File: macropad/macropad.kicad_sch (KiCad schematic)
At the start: 7 parts, among them SW1 SW_Push, SW2 SW_Push, SW3 SW_Push, SW4 SW_Push, U1 XIAO-RP2040-DIP

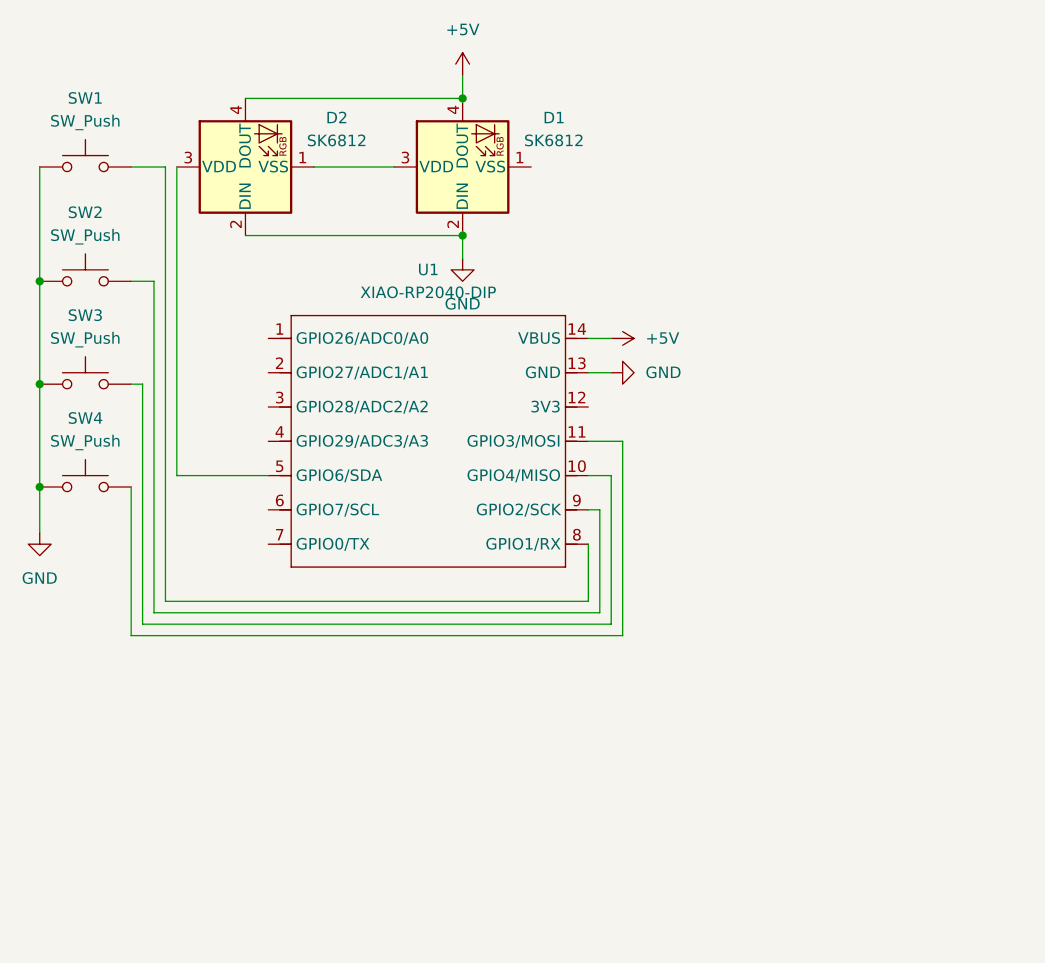
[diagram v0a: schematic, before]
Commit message: Add files via upload
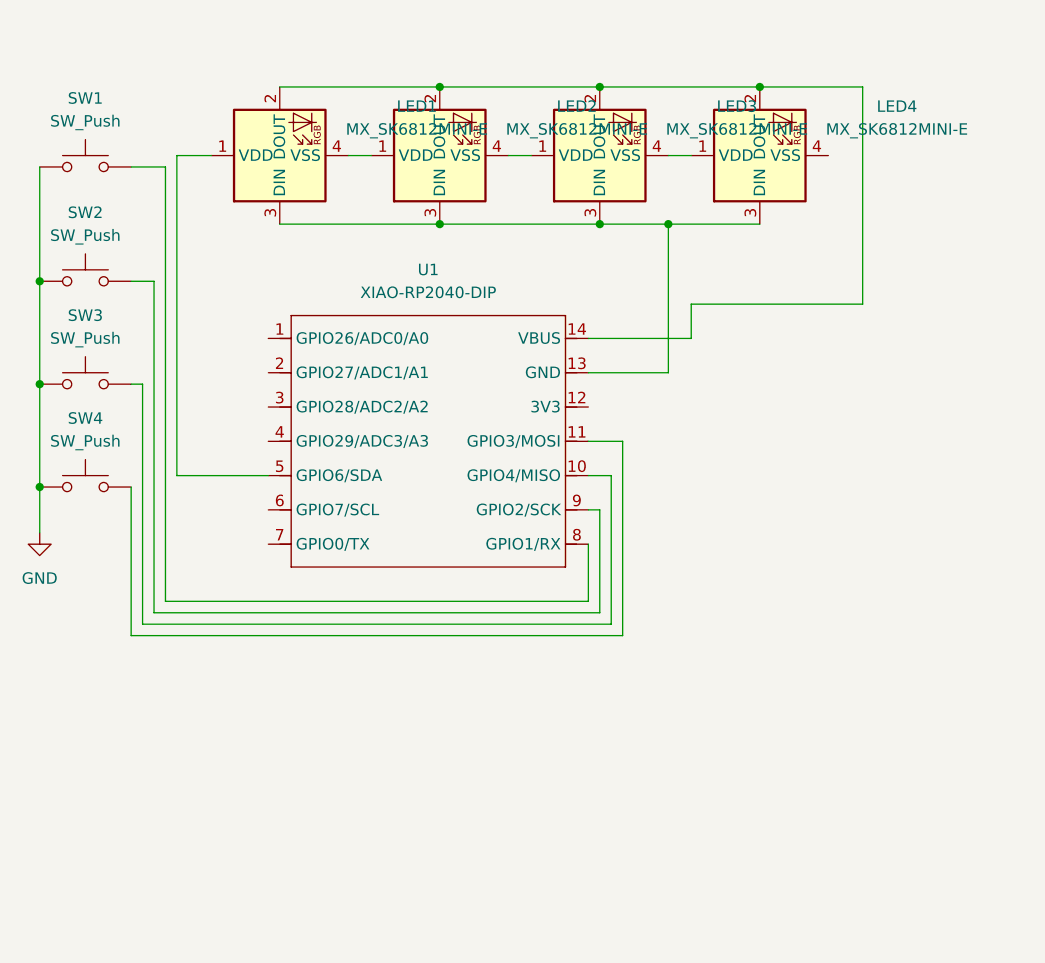
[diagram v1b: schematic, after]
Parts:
- removed D1, D2: SK6812, LED_SMD:LED_SK6812_PLCC4_5.0x5.0mm_P3.2mm, symbol LED:SK6812
- added LED1, LED2, LED3, LED4: MX_SK6812MINI-E, marbastlib-mx:LED_MX_6028R, symbol marbastlib-mx:MX_SK6812MINI-E
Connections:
- net GND: no longer U1.13 (GND)
- net at U1.5 (GPIO6/SDA): now also LED1.1 (VDD)
- net +5V: no longer names the net of U1.14 (VBUS)
- net +5V: now also LED1.2 (DOUT), LED2.2 (DOUT), LED3.2 (DOUT), LED4.2 (DOUT)
- new net: LED1.4 (VSS), LED2.1 (VDD)
- new net: LED1.3 (DIN), LED2.3 (DIN), LED3.3 (DIN), LED4.3 (DIN), U1.13 (GND)
- new net: LED2.4 (VSS), LED3.1 (VDD)
- new net: LED3.4 (VSS), LED4.1 (VDD)

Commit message: Add files via upload
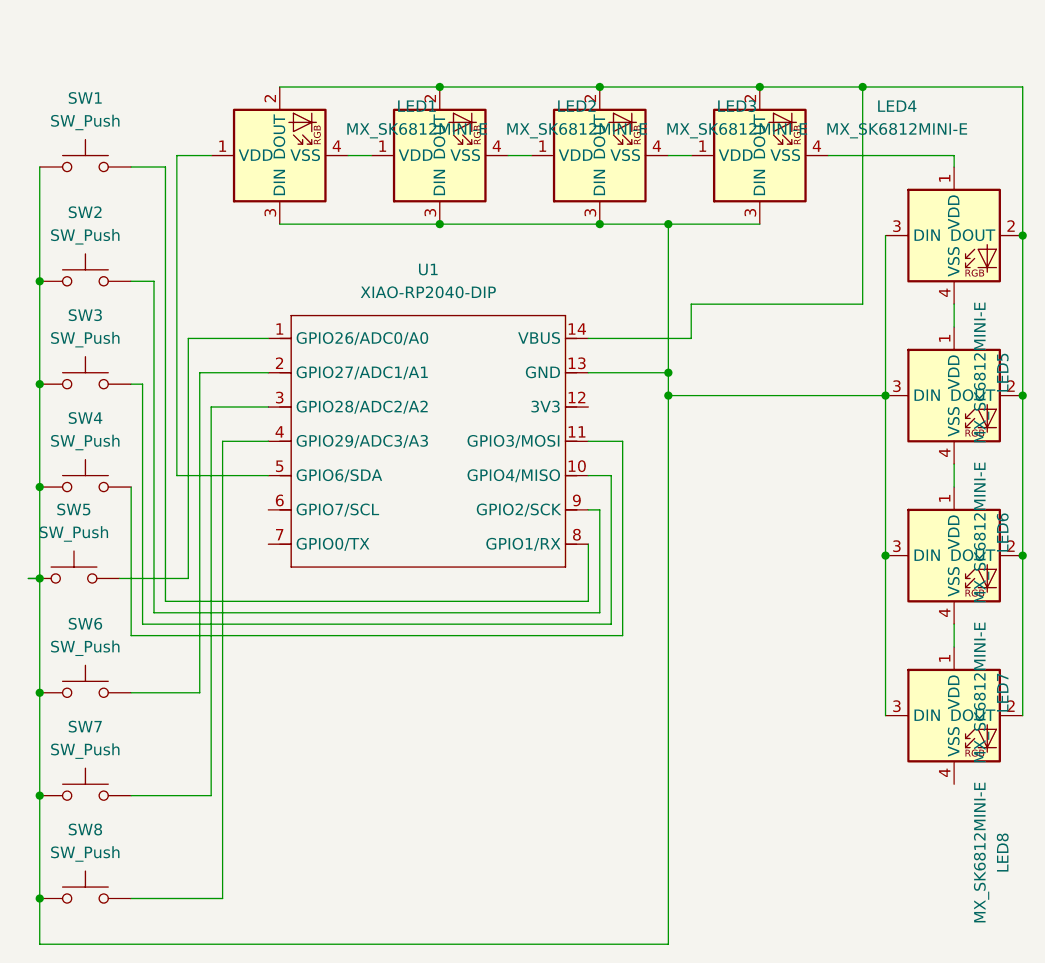
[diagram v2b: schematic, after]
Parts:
- added LED5, LED6, LED7, LED8: MX_SK6812MINI-E, marbastlib-mx:LED_MX_6028R, symbol marbastlib-mx:MX_SK6812MINI-E
- added SW5, SW6, SW7, SW8: SW_Push, Button_Switch_Keyboard:SW_Cherry_MX_1.00u_PCB, symbol Switch:SW_Push
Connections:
- net GND is gone; now on an unnamed net: SW1.1, SW2.1, SW3.1, SW4.1
- net at LED1.2 (DOUT), LED2.2 (DOUT), LED3.2 (DOUT)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: now also LED5.2 (DOUT), LED6.2 (DOUT), LED7.2 (DOUT), LED8.2 (DOUT)
- net at LED1.3 (DIN), LED2.3 (DIN), LED3.3 (DIN)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: now also LED5.3 (DIN), LED6.3 (DIN), LED7.3 (DIN), LED8.3 (DIN), SW5.1, SW6.1, SW7.1, SW8.1
- net at U1.1 (GPIO26/ADC0/A0): now also SW5.2
- net at U1.2 (GPIO27/ADC1/A1): now also SW6.2
- net at U1.3 (GPIO28/ADC2/A2): now also SW7.2
- net at U1.4 (GPIO29/ADC3/A3): now also SW8.2
- net at LED4.4 (VSS): now also LED5.1 (VDD)
- new net: LED6.4 (VSS), LED7.1 (VDD)
- new net: LED7.4 (VSS), LED8.1 (VDD)
- new net: LED5.4 (VSS), LED6.1 (VDD)
